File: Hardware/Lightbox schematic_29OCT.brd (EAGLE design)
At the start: 107.9 x 84.8 mm, 7 parts, among them IC2 7805T, U1 ARDUINOR3-DIMENSION

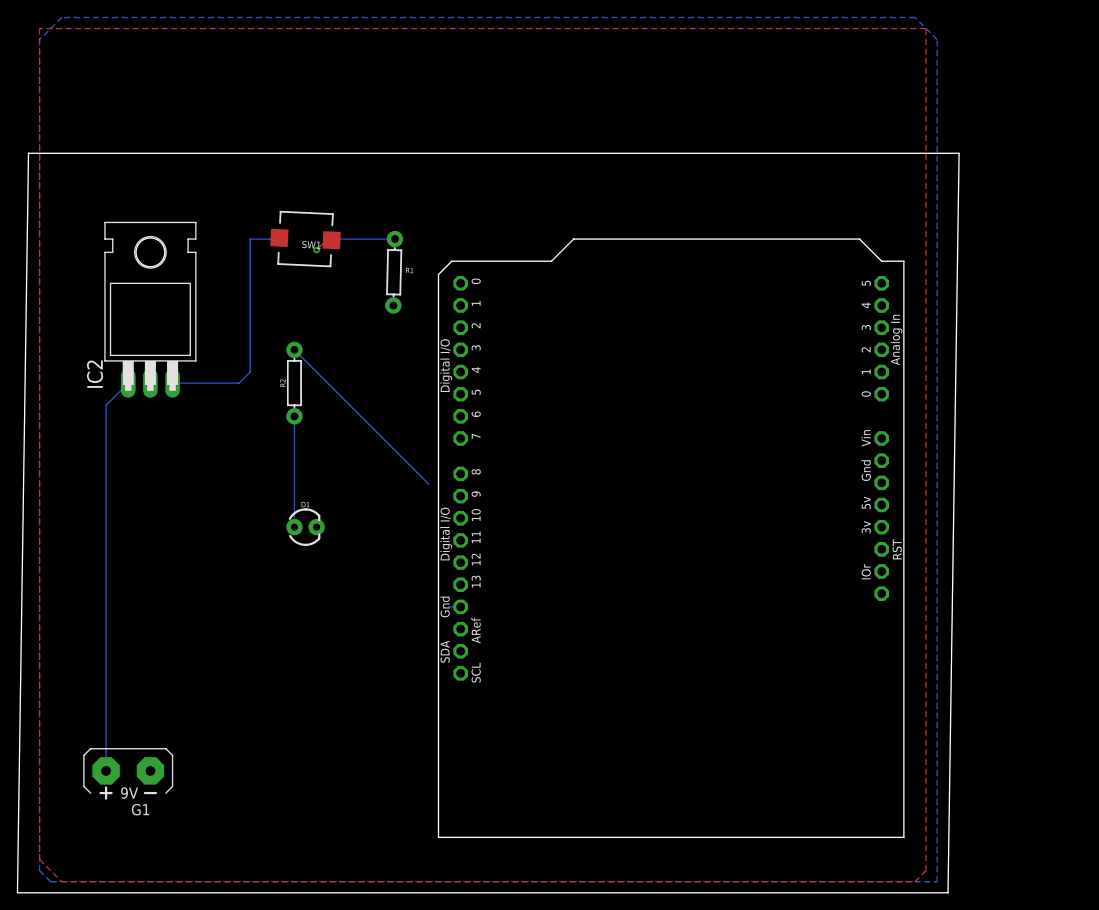
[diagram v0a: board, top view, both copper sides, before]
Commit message: schematic change
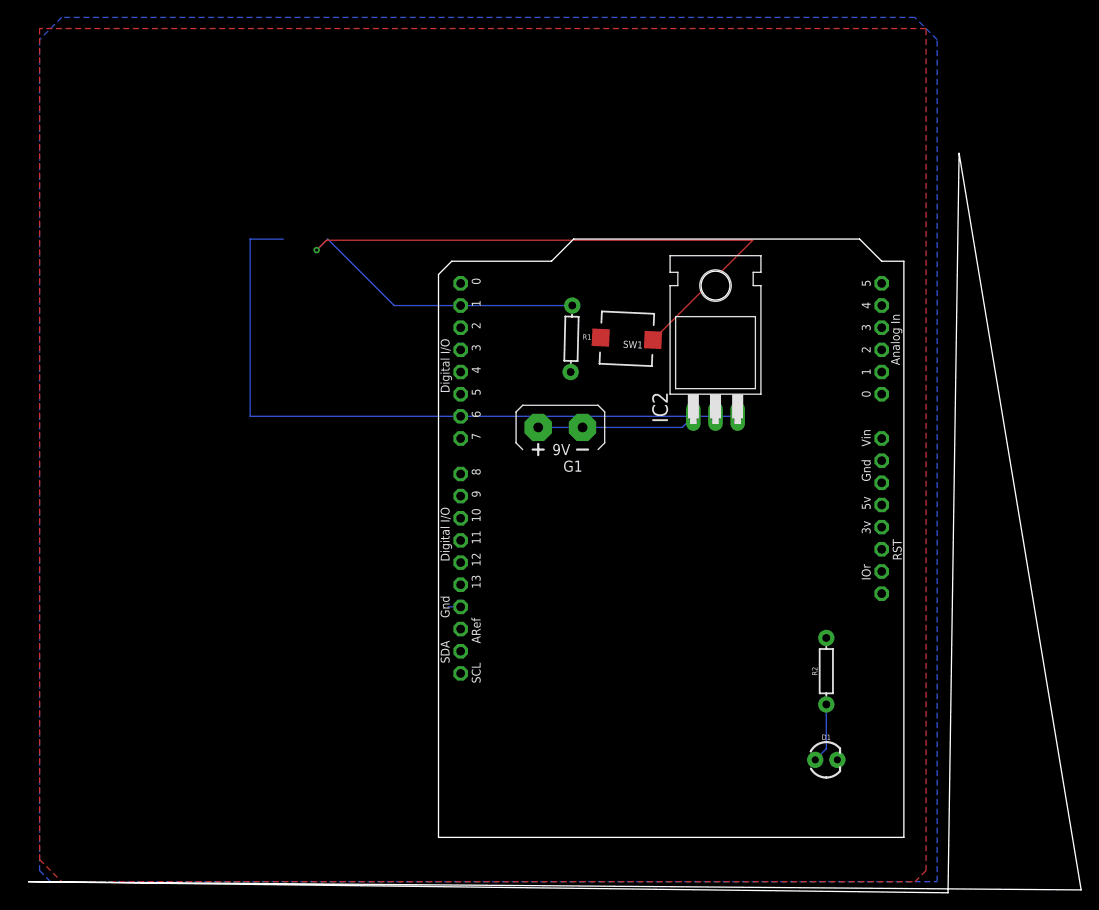
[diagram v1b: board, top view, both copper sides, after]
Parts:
- moved R2 69.3 mm to (92.7, 24.1)
- moved D1 65.4 mm to (92.7, 14.0)
- moved IC2 64.9 mm to (80.0, 63.5)
- moved G1 63.3 mm to (62.2, 52.1)
- moved SW1 38.6 mm to (69.8, 62.2)
- moved R1 21.7 mm to (63.5, 62.2)
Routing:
- net N$2: track 11.7 -> 99.6 mm
- net +5V: track 28.5 -> 80.0 mm
- net N$1: track 45.5 -> 18.3 mm
- net N$3: track 21.8 -> 0.00 mm
- net N$4: track 12.7 -> 6.88 mm
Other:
- board size 107.9 x 84.8 mm -> 120.7 x 84.8 mm
